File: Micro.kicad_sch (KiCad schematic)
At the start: 2 parts, among them U9 STM32L476RGTx

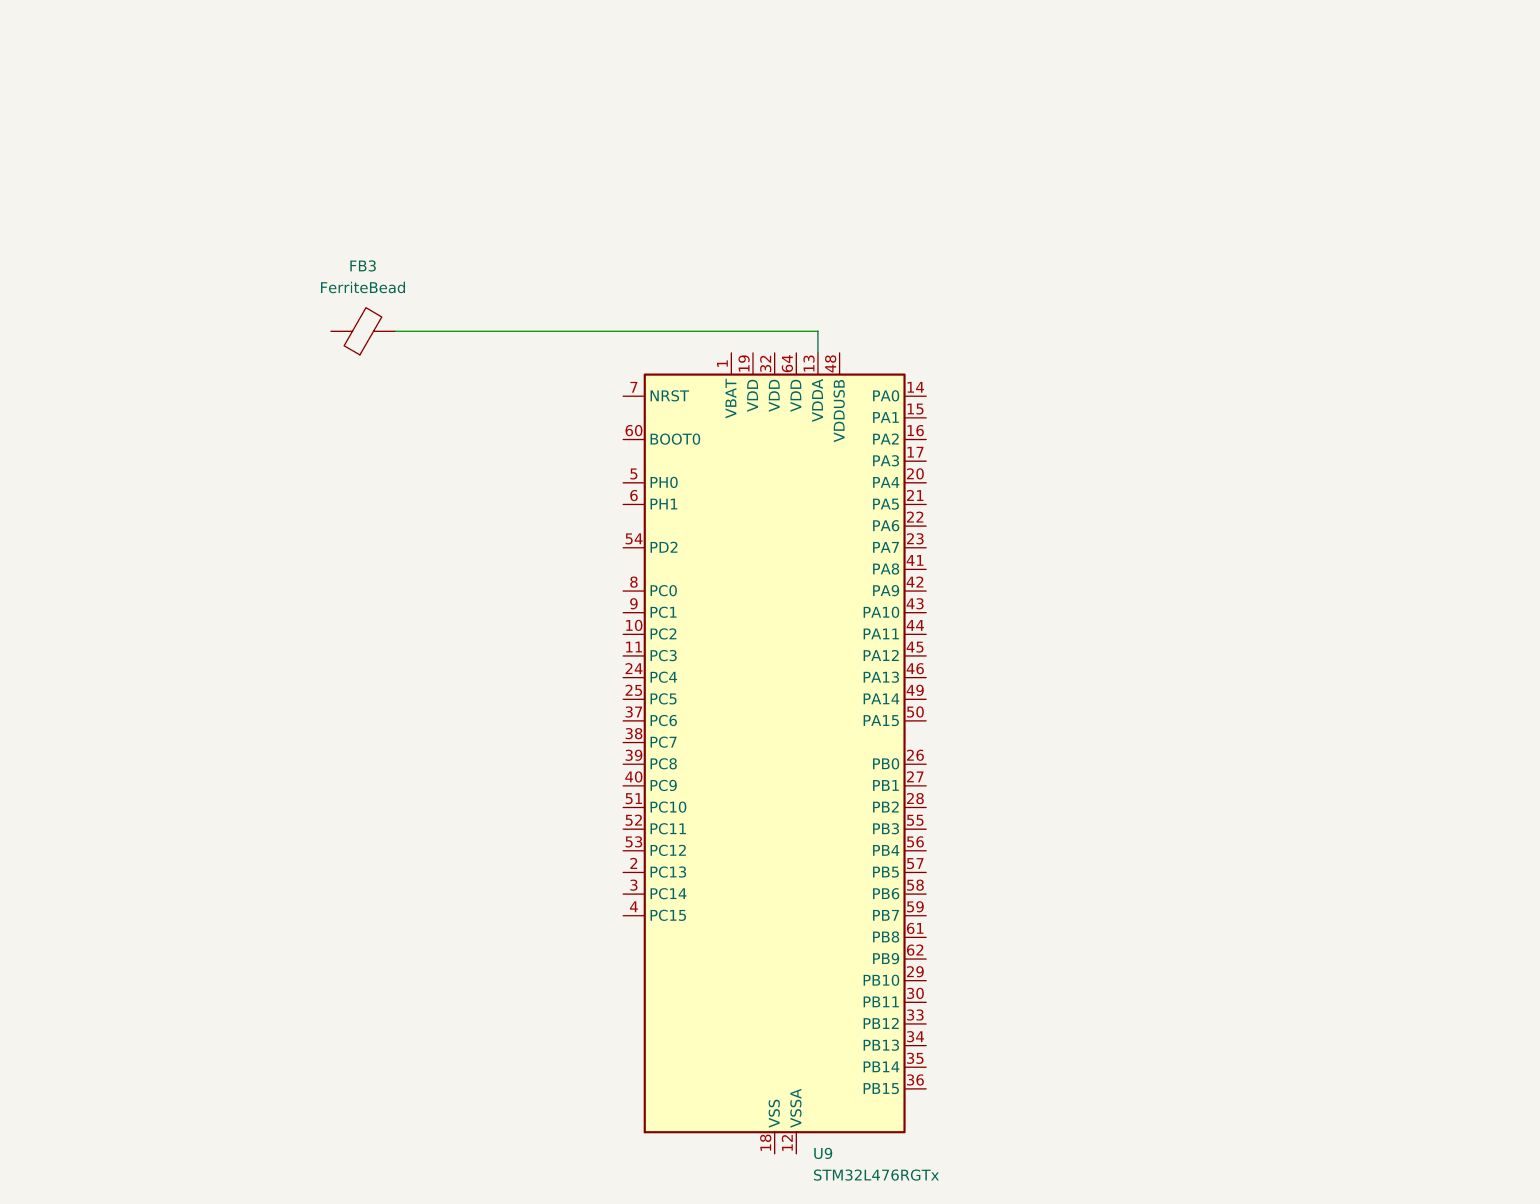
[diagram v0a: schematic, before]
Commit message: Add files via upload
Finished everything except for the micro schematic
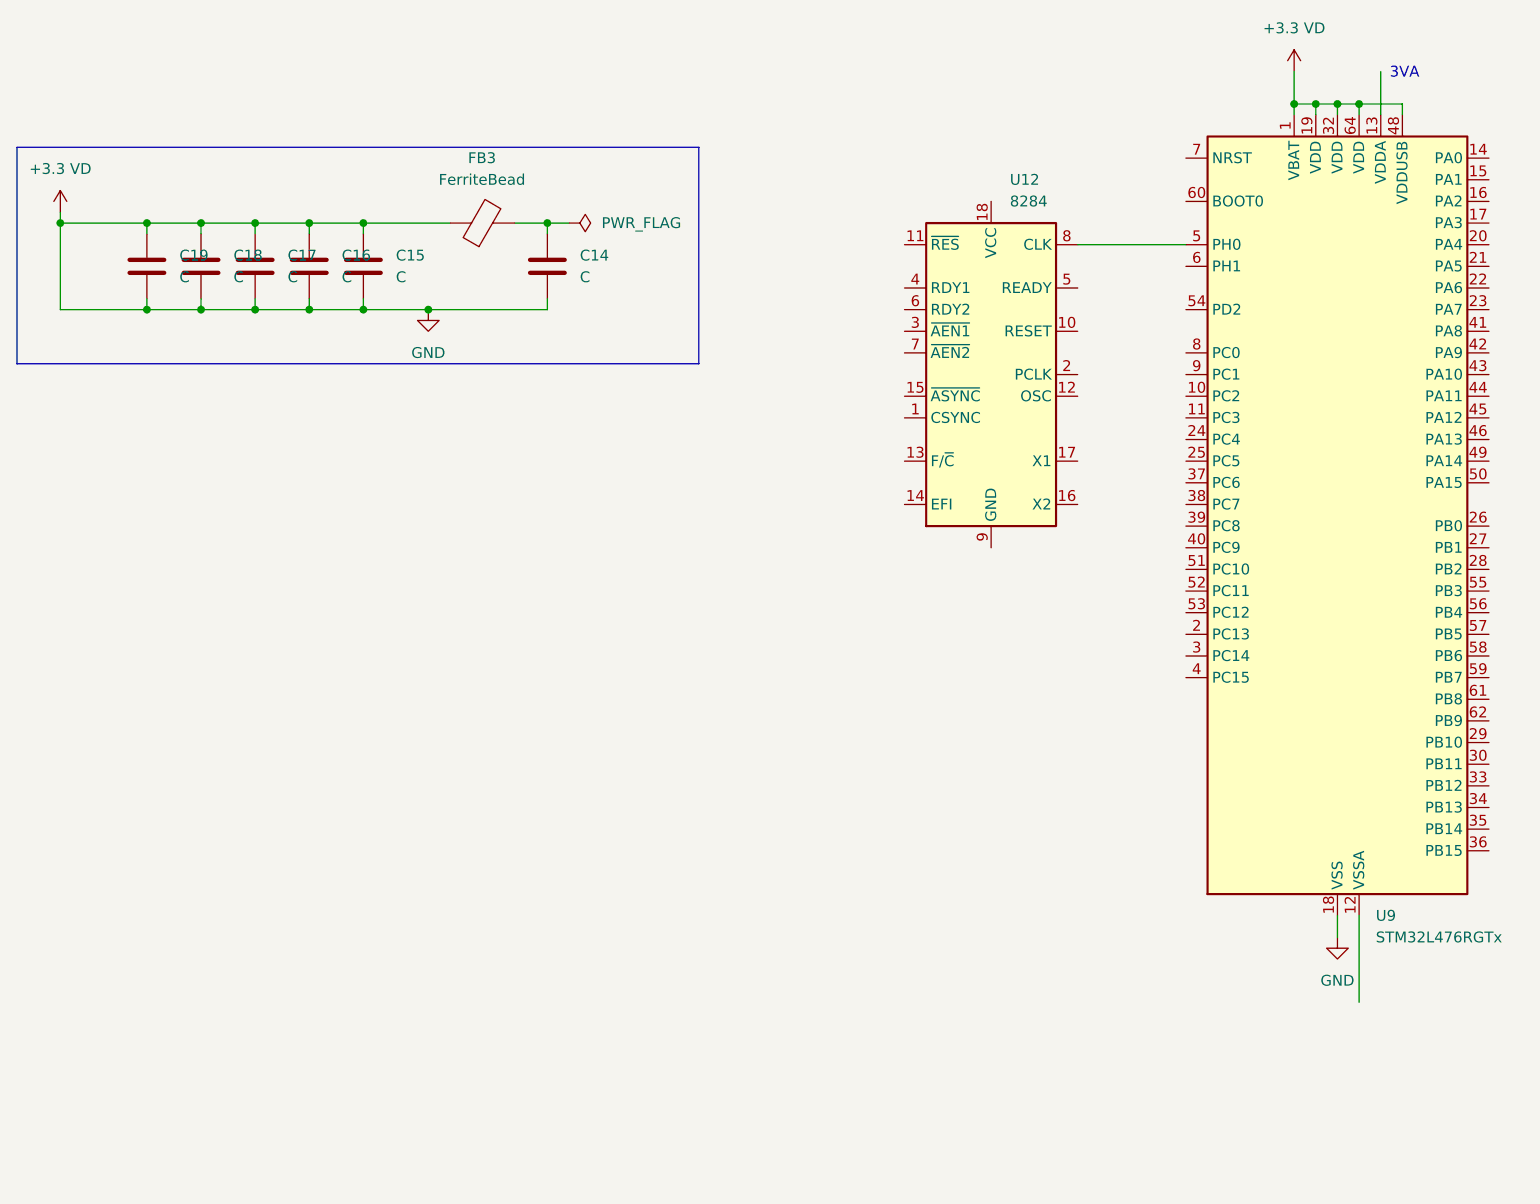
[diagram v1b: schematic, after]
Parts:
- added C14, C15, C16, C17, C18, C19: C, symbol Device:C
- added U12: 8284, Package_DIP:DIP-18_W7.62mm, symbol Timer:8284
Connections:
- net +3.3 VD: now reaches FB3.1
- net +3.3 VD: now also U9.1 (VBAT), U9.18 (VSS), U9.19 (VDD), U9.31 (VSS), U9.32 (VDD), U9.47 (VSS), U9.48 (VDDUSB), U9.63 (VSS), U9.64 (VDD), C14.2, C15.1, C15.2, C16.1, C16.2, C17.1, C17.2, C18.1, C18.2, C19.1, C19.2
- net at FB3.2: now also C14.1; no longer U9.13 (VDDA)
- net at U9.5 (PH0): now also U12.8 (CLK)
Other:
- note added: "3VA"
- moved on the sheet: FB3, U9
